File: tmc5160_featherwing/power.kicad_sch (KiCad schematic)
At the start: 1 part, among them J1 Conn_01x02_P1.5MM_Molex_Pico-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

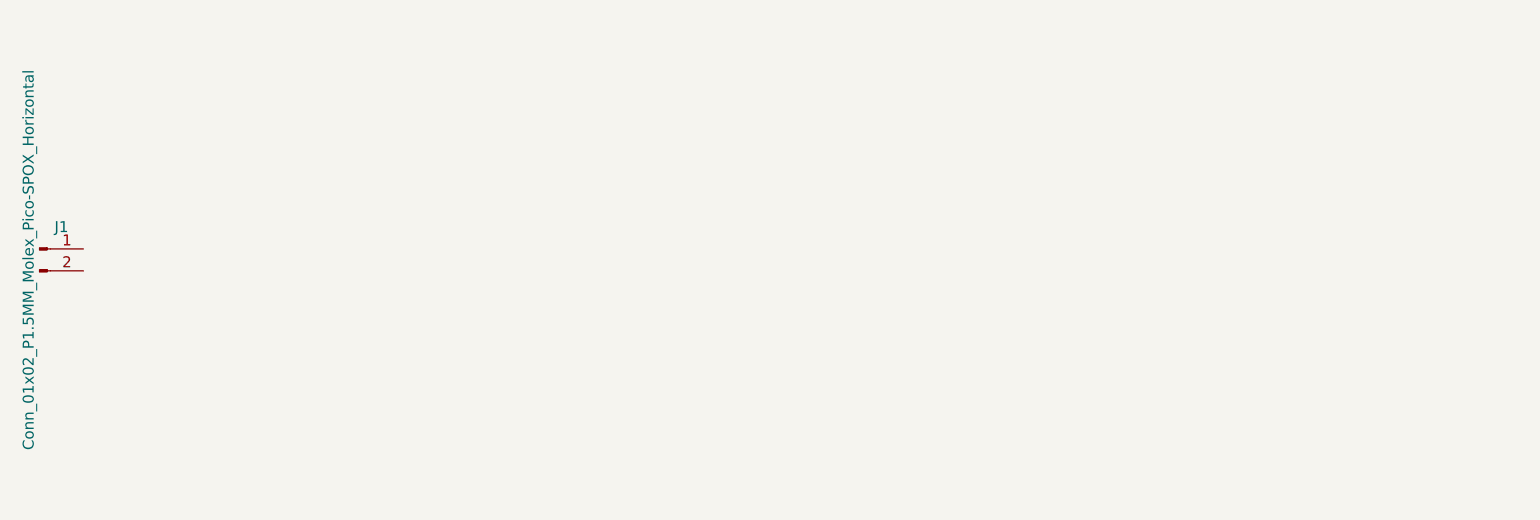
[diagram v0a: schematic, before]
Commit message: Add to power sheet
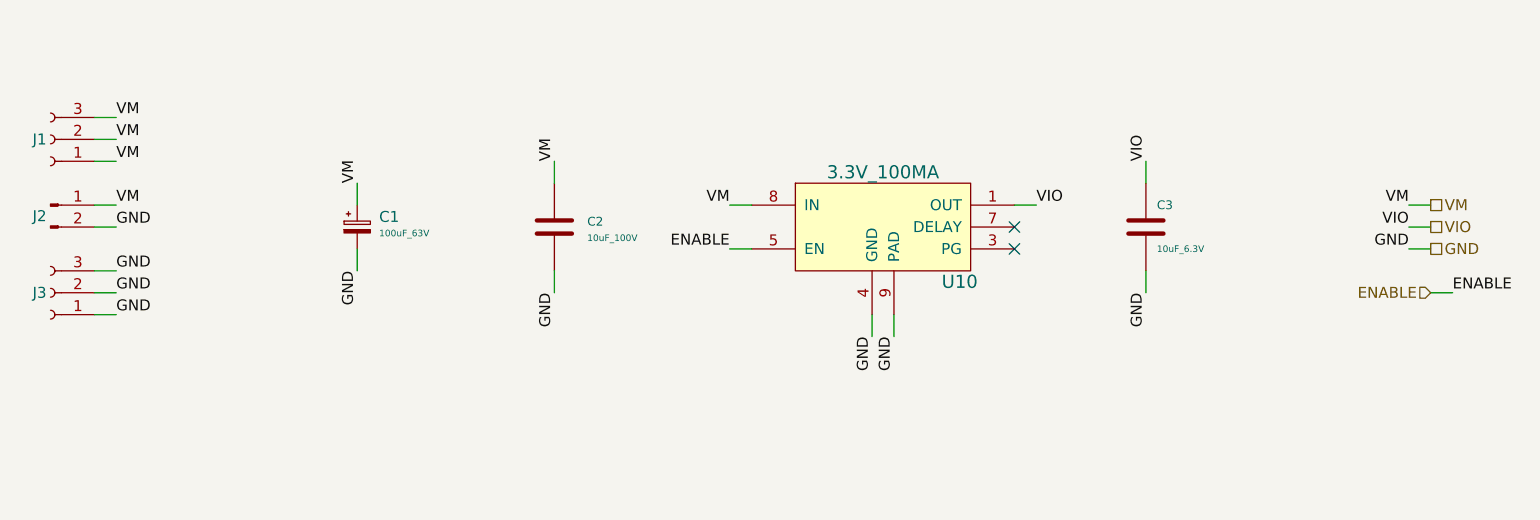
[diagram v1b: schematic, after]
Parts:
- removed J1: Conn_01x02_P1.5MM_Molex_Pico-SPOX_Horizontal, Janelia:Molex_Pico-SPOX_87438_1x02-P1.5MM_Horizontal, symbol Janelia:Conn_01x02_P1.5MM_Molex_Pico-SPOX_Horizontal
- added C1: 100uF_63V, Janelia:CP_Elec_10x10.5, symbol Janelia:CP_100uF_63V_10x10.5MM
- added C2: 10uF_100V, Janelia:C_1210_3225Metric, symbol Janelia:C_10uF_100V_1210
- added C3: 10uF_6.3V, Janelia:C_0402_1005Metric, symbol Janelia:C_10uF_6.3V_0402
- added J1, J3: Conn_01x03_P2.54MM_HeaderHoles, Janelia:PinHeader_1x03_P2.54mm_Vertical_Holes, symbol Janelia:Conn_01x03_P2.54MM_HeaderHoles
- added J2: Conn_01x02_P1.5MM_Molex_Pico-SPOX-87438_Horizontal, Janelia:Molex_Pico-SPOX-87438_1x02-P1.5MM_Horizontal, symbol Janelia:Conn_01x02_P1.5MM_Molex_Pico-SPOX-87438_Horizontal
- added U10: 3.3V_100MA, Janelia:DRB0008B, symbol Janelia:Regulator_Linear_3.3V_100MA_60Vin
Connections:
- new net ENABLE: U10.5 (EN)
- new net GND: C1.2, C2.2, C3.2, J2.2 (Pin_2), J3.1 (Pin_1), J3.2 (Pin_2), J3.3 (Pin_3), U10.4 (GND), U10.9 (PAD)
- new net VIO: C3.1, U10.1 (OUT)
- new net VM: C1.1, C2.1, J1.1 (Pin_1), J1.2 (Pin_2), J1.3 (Pin_3), J2.1 (Pin_1), U10.8 (IN)
- no-connect marks 0 -> 2
